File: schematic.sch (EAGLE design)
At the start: 31 parts, among them IC1 FT230XS, IC2 ATMEGA644A, IC4 L4931D, X1 MINI-USB-32005-301

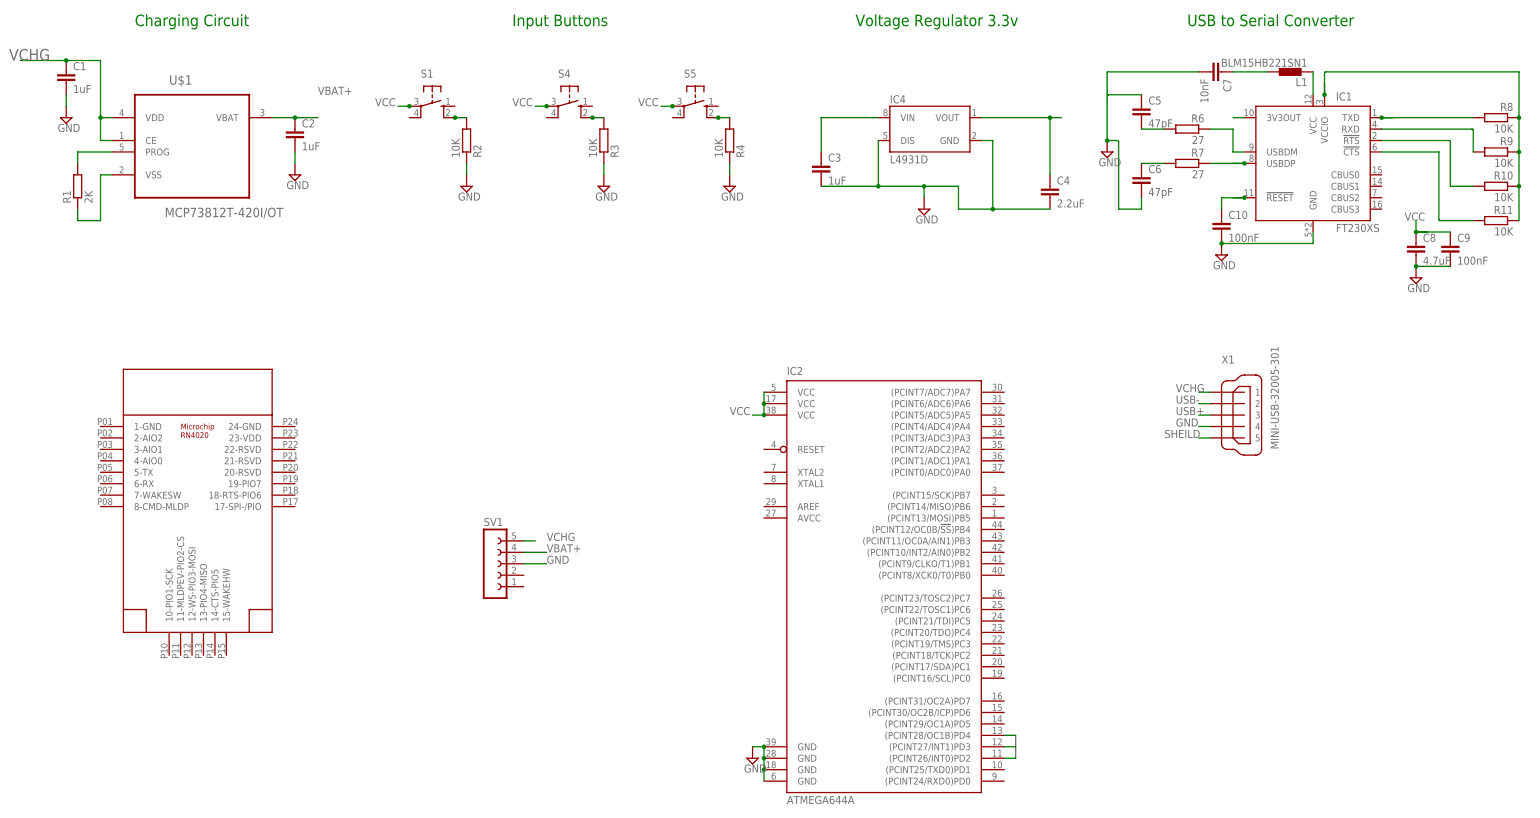
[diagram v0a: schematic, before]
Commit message: saving to git
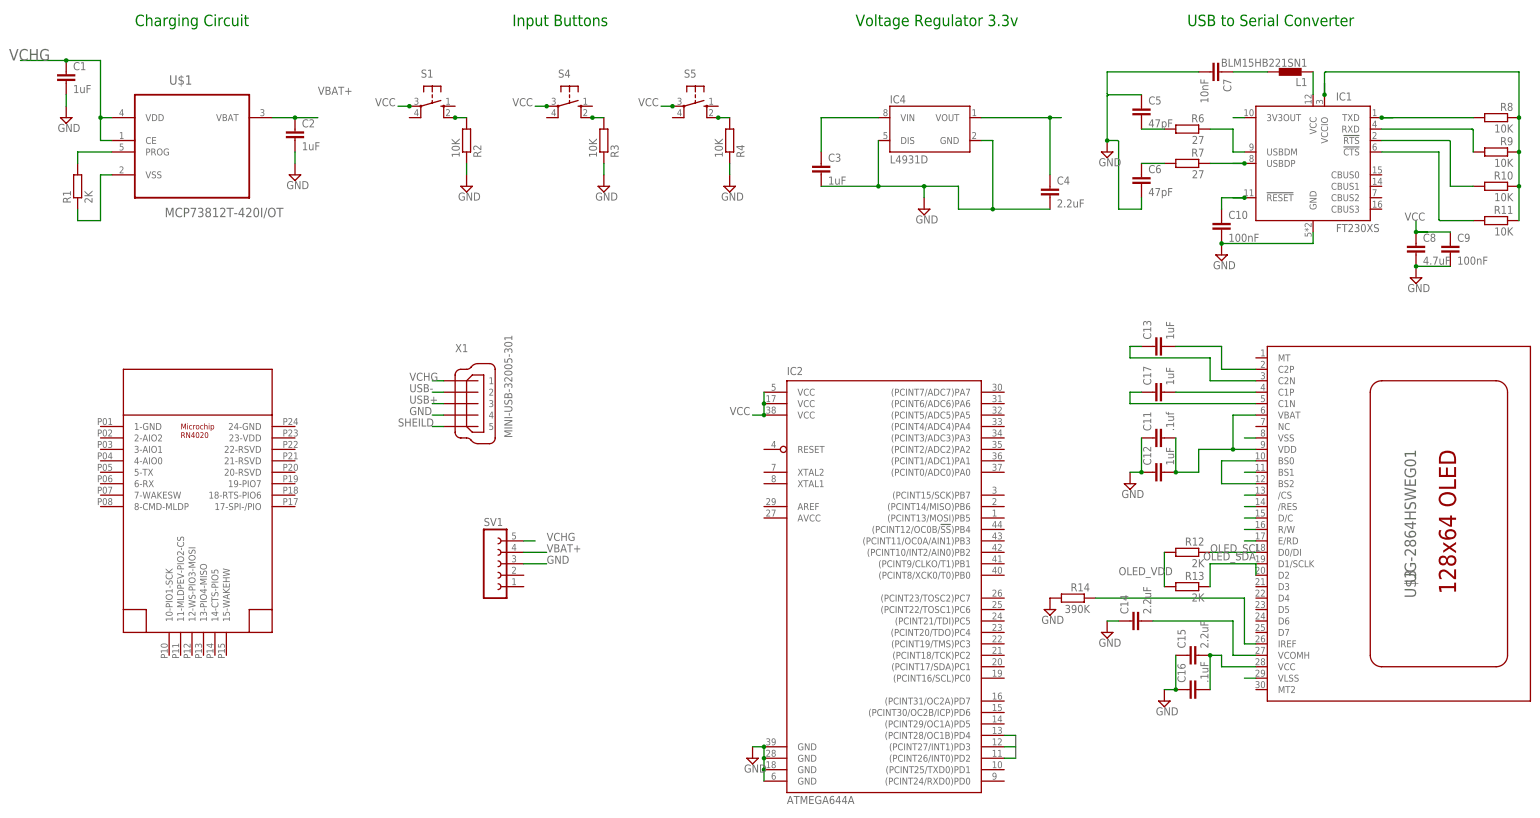
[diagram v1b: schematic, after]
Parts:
- added C11: .1uf, eagle-ltspice:CC0504
- added C12, C13, C17: 1uF, eagle-ltspice:CC0504
- added C14, C15: 2.2uF, eagle-ltspice:CC0504
- added C16: .1uF, eagle-ltspice:CC0504
- added R12, R13: 2K, eagle-ltspice:RR0603
- added R14: 390K, eagle-ltspice:RR0603
- added U$3: UG-2864HSWEG01, adafruit:UG-2864HSWEG01
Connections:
- new net N$10: C13.1, U$3.C2N
- new net N$11: C17.2, U$3.C1P
- new net N$12: C17.1, U$3.C1N
- new net N$5: C14.2, U$3.VCOMH
- new net N$7: C13.2, U$3.C2P
- new net N$9: R14.1, U$3.IREF
- new net OLED_SCL: R12.1, U$3.D0/DI
- new net OLED_SDA: R13.1, U$3.D1/SCLK, U$3.D2
- new net OLED_VCC: C15.2, C16.2, U$3.VCC
- new net OLED_VDD: C11.2, C12.2, R12.2, R13.2, U$3./RES, U$3.BS1, U$3.VBAT, U$3.VDD
- new net OLED_VSS: U$3./CS, U$3.BS0, U$3.BS2, U$3.R/W
- net GND: now also C11.1, C12.1, C14.1, C15.1, C16.1, R14.2, U$3.D/C, U$3.E/RD, U$3.VLSS, U$3.VSS
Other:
- moved on the sheet: X1
